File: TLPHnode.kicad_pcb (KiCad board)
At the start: 4 copper layers, 28 x 20.5 mm, 29 parts, among them P1 Bat, P2 CONN_01X05, SW1 Reset, U1 NCP703, U2 LD39130S, U3 LPS25HB, U4 Si7006-A20, U5 ESP-12E, U6 ISL29035

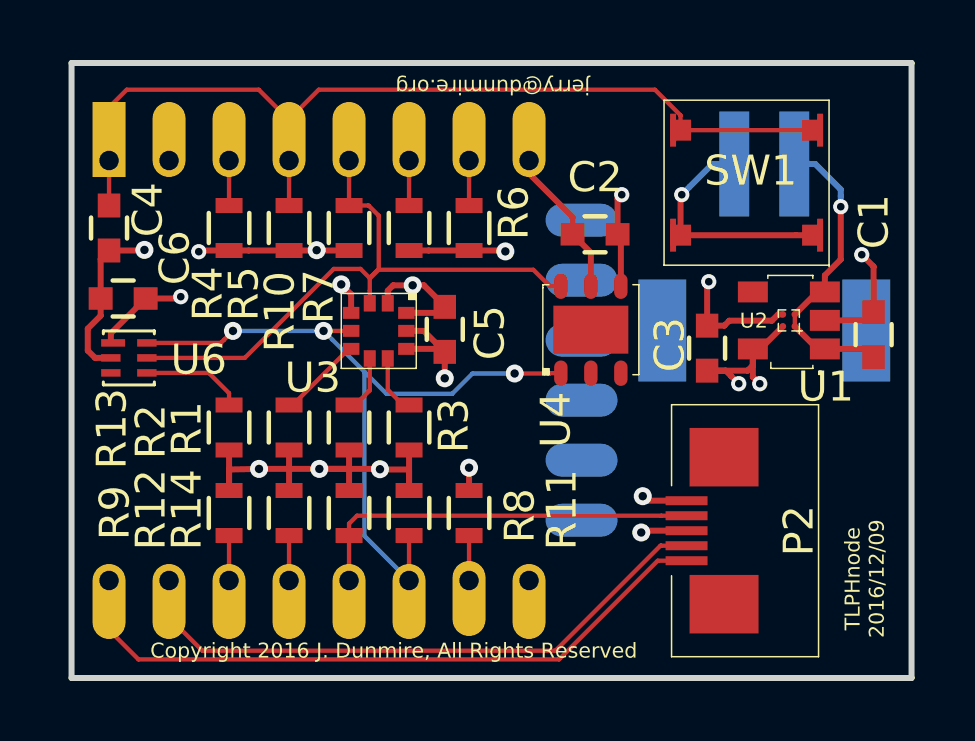
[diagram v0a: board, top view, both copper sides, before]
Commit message: Add Logo
On branch master
modified:   TLPHnode.kicad_pcb
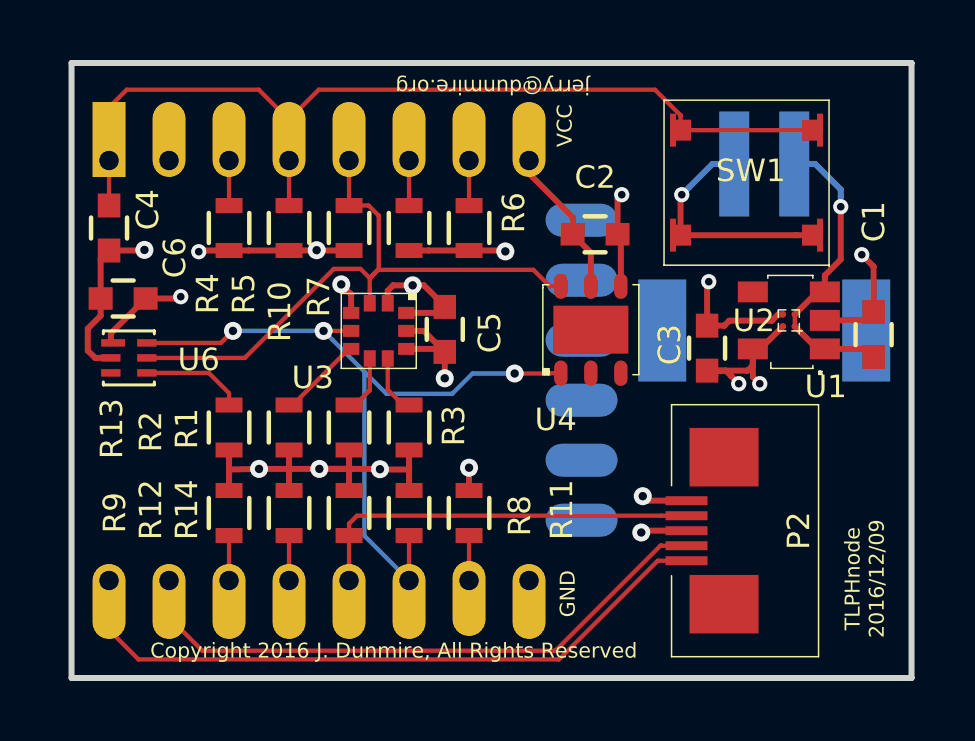
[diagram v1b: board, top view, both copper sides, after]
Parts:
- added Ref**: RockingDLogo_9x7, rockingDLogos:RockingDLogo_9x7, B.Cu at (157.8, 96.0)
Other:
- board text added: "GND"
- board text added: "VBat"
- board text added: "VCC"
